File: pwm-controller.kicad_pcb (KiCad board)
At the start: 2 copper layers, 50 x 50 mm, 75 parts, among them J2 OUT-, J4 POWER, J5 OUT+, J6 DEBUG, J7 I2C, Q1 AO3400A, Q10 MMBT5551, Q11 MMBT5551, Q12 MMBT5401, Q2 AO3400A, Q3 AO3400A, Q4 AO3400A, Q5 AO3400A, Q6 AO3400A, Q7 MMBT5551, Q8 MMBT5551, Q9 MMBT5401, SW1 EC12D1524403, U1 L78L09_SOT89, U3 STM8S003F3Px, U4 HT7533-1-SOT89

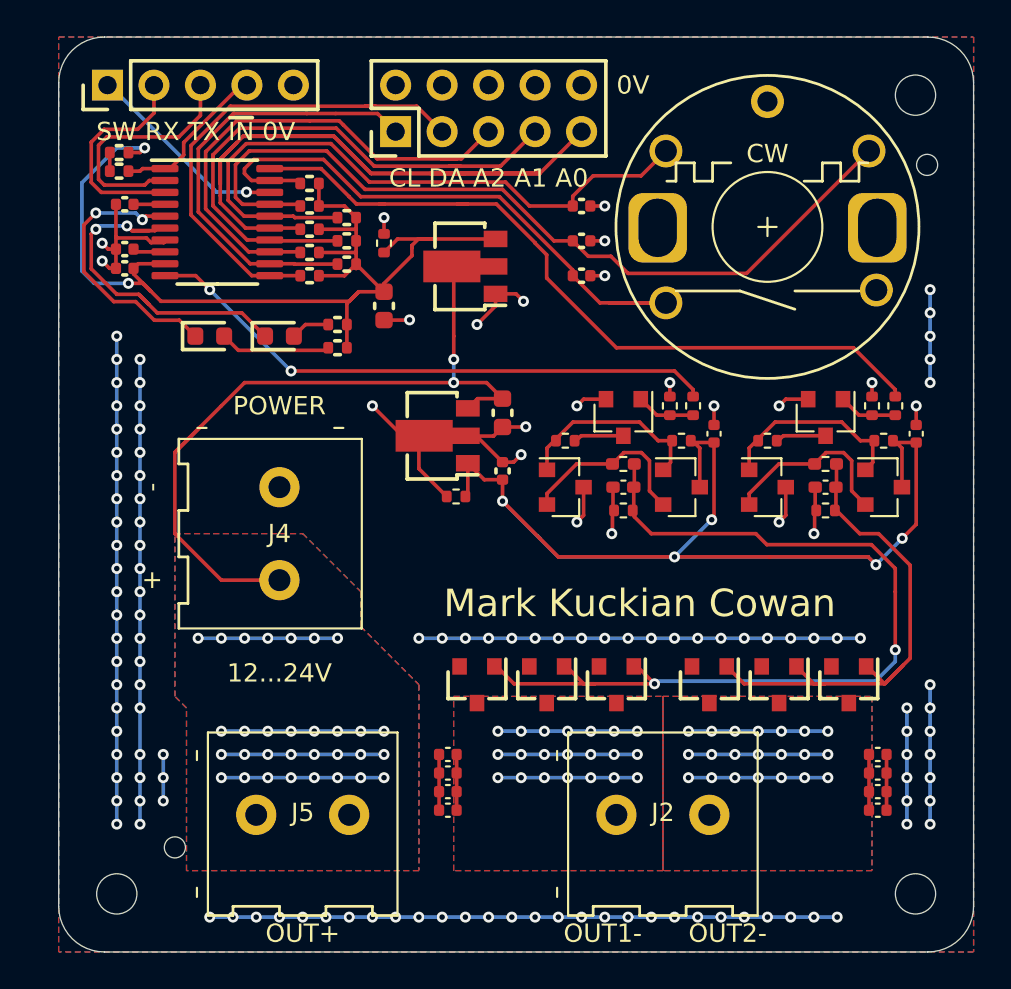
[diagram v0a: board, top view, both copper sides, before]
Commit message: ready?
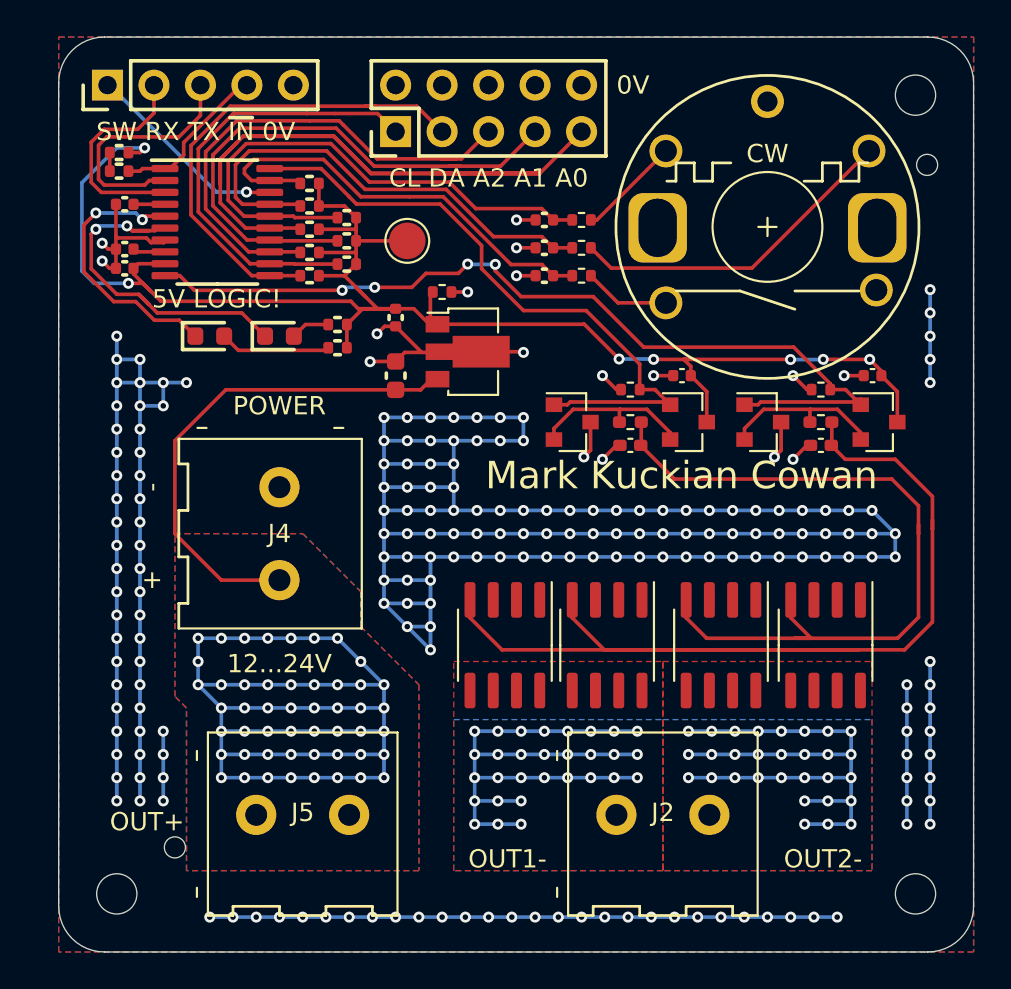
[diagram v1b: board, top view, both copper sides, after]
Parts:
- removed C13, C14, C15, C16, C17, C18, C19, C20: 100n/50, Capacitor_SMD:C_0402_1005Metric
- removed C9: 1u/50, Capacitor_SMD:C_0603_1608Metric
- removed Q11, Q8: MMBT5551, Package_TO_SOT_SMD:SOT-23
- removed Q3, Q6: AO3400A, Package_TO_SOT_SMD:SOT-23
- removed R18, R23, R25, R27: 4.7k, Resistor_SMD:R_0402_1005Metric
- removed R19, R28: 1k, Resistor_SMD:R_0402_1005Metric
- removed U4: HT7533-1-SOT89, Package_TO_SOT_SMD:SOT-89-3
- added TP1: TP5V, TestPoint:TestPoint_Pad_D2.0mm, F.Cu at (95.2, 87.3)
- C3, C4: value 100n/50 -> 3.3n
- Q1, Q2, Q4, Q5: value AO3400A -> NTMS4807; footprint Package_TO_SOT_SMD:SOT-23 -> mark:NTMS-4807N-SOIC-8-3.9x4.9x1.27P
- R1, R17, R3: value 4.7k -> 220
- R15, R16: value 120 -> 220
- R2, R24: value 120 -> 4.7k
- U1: value L78L09_SOT89 -> 78L05
- moved R1 20.4 mm to (104.8, 86.2)
- moved R3 13.6 mm to (104.8, 89.2)
- moved R20 13.2 mm to (107.4, 95.5), turned to 180 degrees
- moved C10 13.2 mm to (110.3, 94.7), turned to 180 degrees
- moved Q10 11.4 mm to (121.0, 97.2)
- moved Q12 11.4 mm to (114.7, 97.2)
- moved Q9 11.2 mm to (104.3, 97.2)
- moved Q7 11.2 mm to (110.6, 97.2)
- moved R12 11.2 mm to (97.2, 90.1), turned to 180 degrees
- moved C4 11.0 mm to (117.9, 98.5)
- moved R24 11.0 mm to (117.9, 97.2)
- moved C3 10.9 mm to (107.4, 98.5)
- moved R2 10.9 mm to (107.4, 97.2)
- moved R17 10.8 mm to (104.8, 87.7), turned to 180 degrees
- moved C2 10.2 mm to (94.6, 91.5), turned to 270 degrees
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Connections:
- C10 pad 1: +9V -> +5V
- C2 pad 1: +9V -> +5V
- C5 pad 1: +9V -> +5V
- C8 pad 2: +3V3 -> +5V
- Q10 pad 1: Net-(Q10-Pad1) -> PWM2
- Q10 pad 3: +9V -> +5V
- Q12 pad 1: Net-(Q10-Pad1) -> PWM2
- Q7 pad 1: Net-(Q7-Pad1) -> PWM1
- Q7 pad 3: +9V -> +5V
- Q9 pad 1: Net-(Q7-Pad1) -> PWM1
- R1 pad 1: +9V -> Net-(R1-Pad1)
- R1 pad 2: Net-(Q7-Pad1) -> RE_I
- R10 pad 2: +3V3 -> +5V
- R11 pad 2: +3V3 -> +5V
- R12 pad 2: +9V -> +5V
- R14 pad 2: +3V3 -> +5V
- R15 pad 2: +3V3 -> +5V
- R16 pad 2: +3V3 -> +5V
- R17 pad 1: GND -> Net-(R17-Pad1)
- R17 pad 2: +3V3 -> RE_Q
- R20 pad 1: Net-(Q8-Pad1) -> PWM1
- R29 pad 1: Net-(Q11-Pad1) -> PWM2
- R3 pad 1: Net-(Q7-Pad1) -> RE_B
- R3 pad 2: Net-(Q8-Pad3) -> Net-(R3-Pad2)
- R4 pad 2: +3V3 -> +5V
- R5 pad 2: +3V3 -> +5V
- R6 pad 2: +3V3 -> +5V
- R7 pad 2: +3V3 -> +5V
- R8 pad 2: +3V3 -> +5V
- R9 pad 2: +3V3 -> +5V
- SW1 pad A: RE_I -> Net-(R1-Pad1)
- SW1 pad B: RE_Q -> Net-(R17-Pad1)
- SW1 pad S1: RE_B -> Net-(R3-Pad2)
- U1 pad 1: +9V -> +5V
- U3 pad 9: +3V3 -> +5V
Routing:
- net GND: track 190.3 -> 290.9 mm, vias 133 -> 212
- net +5V: track 0.00 -> 91.7 mm, vias 0 -> 7
- net +9V: track 71.7 -> 0.00 mm, vias 5 -> 0
- net +3V3: track 60.0 -> 0.00 mm, vias 2 -> 0
- net VIN: track 77.6 -> 97.3 mm, vias 33 -> 50
- net RE_Q: track 46.0 -> 26.4 mm
- net Net-(R17-Pad1): track 0.00 -> 18.3 mm
- net PWM2: track 31.8 -> 49.3 mm, vias 2 -> 4
- net /channel1/GATE: track 28.6 -> 42.5 mm
- net DRAIN1: track 25.9 -> 36.8 mm, vias 21 -> 30
- net DRAIN2: track 25.9 -> 36.8 mm, vias 21 -> 30
- net /channel2/GATE: track 49.4 -> 60.3 mm, vias 2 -> 0
- net Net-(Q7-Pad1): track 10.7 -> 0.00 mm
- net Net-(Q10-Pad1): track 10.7 -> 0.00 mm
- net RE_B: track 33.3 -> 24.3 mm
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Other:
- board text removed: "10A should cause up to 100mV noise on GND. Slotting GND plane to reduce noise in digital section."
